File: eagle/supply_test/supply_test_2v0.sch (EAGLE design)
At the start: 53 parts, among them J1 SOCKET, J10 SOCKET, J11 SOCKET, J12 SOCKET, J13 SOCKET, J14 SOCKET, J15 SOCKET, J16 SOCKET, J17 SOCKET, J18 SOCKET, J19 SOCKET, J2 SOCKET, J20 SOCKET, J21 AC_INSW, J22 SOCKET, J3 SOCKET, J4 SOCKET, J5 SOCKET, J6 SOCKET, J7 SOCKET, J8 SOCKET, J9 SOCKET, Q1 2N7002, U1 TPS62122

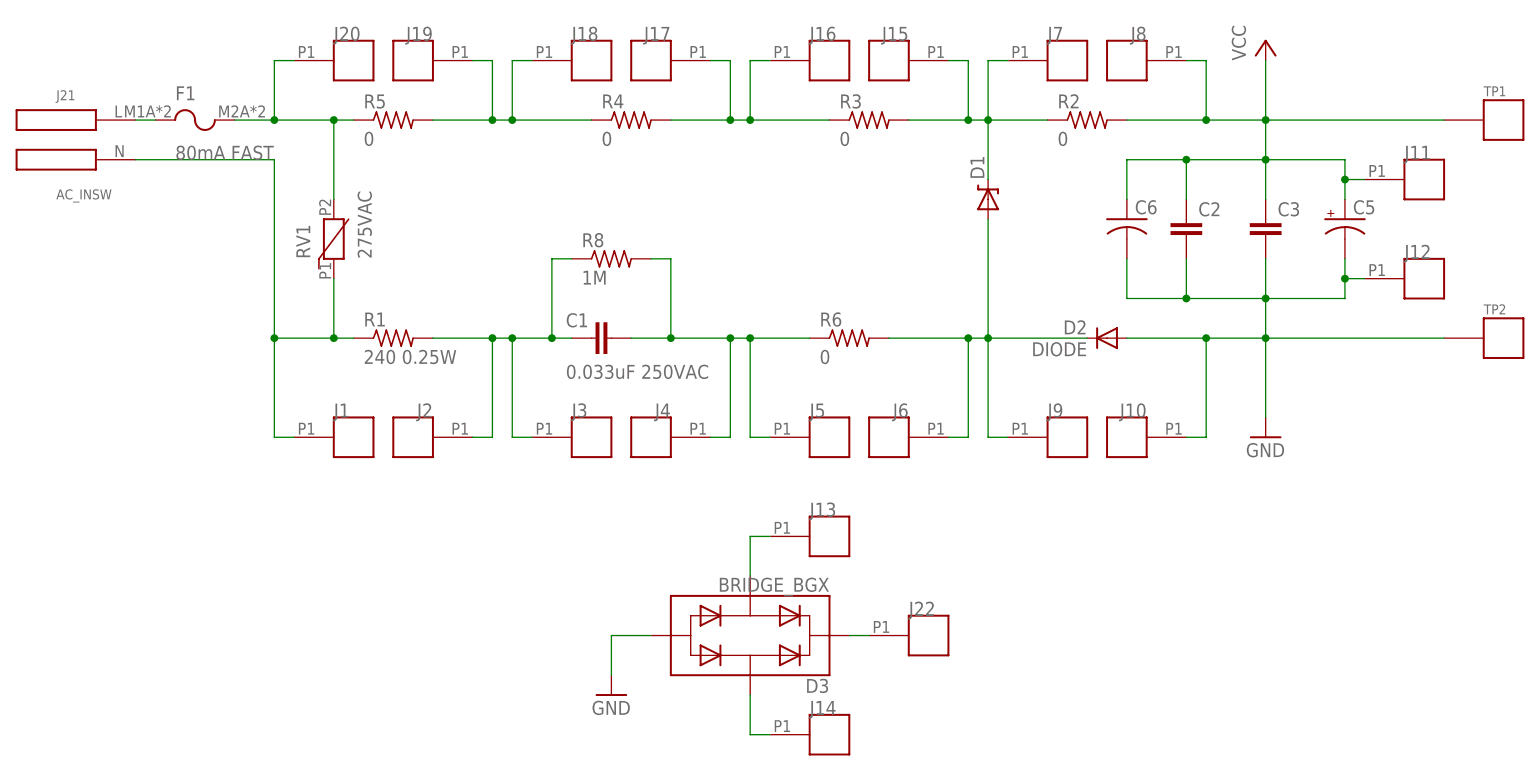
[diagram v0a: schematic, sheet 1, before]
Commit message: miniaturized power supply
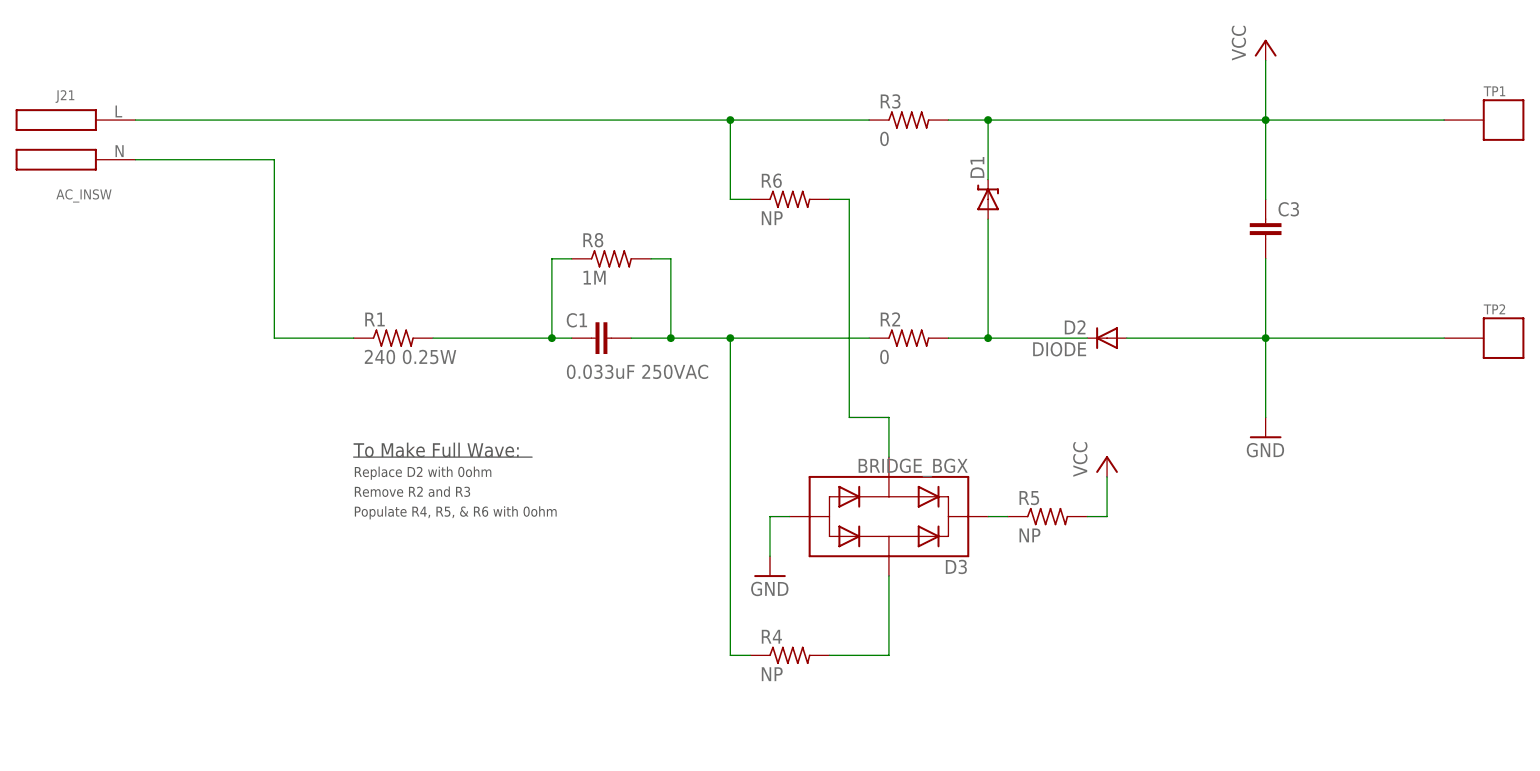
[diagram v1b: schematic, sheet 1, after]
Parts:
- removed C2: (no value), rcl:C-EUC0805
- removed C5: (no value), SparkFun-Passives:CAP_POL1206
- removed C6: (no value), rcl:C-USC1210
- removed F1: 80mA FAST, powerfilm:FUSE
- removed J1, J10, J11, J12, J13, J14, J15, J16, J17, J18, J19, J2, J20, J22, J3, J4, J5, J6, J7, J8, J9: SOCKET, powerfilm:SOCKET
- removed RV1: 275VAC, powerfilm:MOV_CU4032
- R2, R3: DIGIKEY P0.0GCT-ND -> (none)
- R4, R5, R6: value 0 -> NP; DIGIKEY P0.0GCT-ND -> (none)
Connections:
- removed net N$11: F1.P1, J21.P
- removed net N$12: J16.P1, J17.P1, R3.1, R4.2
- removed net N$14: F1.P2, J20.P1, R5.1, RV1.P2
- removed net N$15: J18.P1, J19.P1, R4.1, R5.2
- net GND: no longer C2.2, C5.-, C6.2, J10.P1, J12.P1
- net N$1: no longer J2.P1, J3.P1
- net N$2: no longer J1.P1, RV1.P1
- net N$3: now also D1.A, D2.C, R2.2; no longer C1.1, J4.P1, J5.P1, R6.1, R8.2
- net N$4: now also C1.1, R2.1, R4.1, R8.2; no longer D1.A, D2.C, J6.P1, J9.P1, R6.2
- net N$5: now also D3.P4, R4.2; no longer D1.C, J15.P1, J7.P1, R2.1, R3.2
- net N$6: now also J21.P, R3.1, R6.1; no longer D3.P2, J13.P1
- net N$7: now also R5.1; no longer J22.P1
- net N$8: now also D3.P2, R6.2; no longer D3.P4, J14.P1
- net VCC: now also D1.C, R3.2, R5.2; no longer C2.1, C5.+, C6.1, J11.P1, J8.P1, R2.2
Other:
- note added: "Populate R4, R5, & R6 with 0ohm"
- note added: "Remove R2 and R3"
- note added: "Replace D2 with 0ohm"
- note added: "To Make Full Wave:"
- moved on the sheet: D3, R2, R3, R4, R5, R6
